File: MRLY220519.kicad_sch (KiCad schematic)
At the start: 2 parts

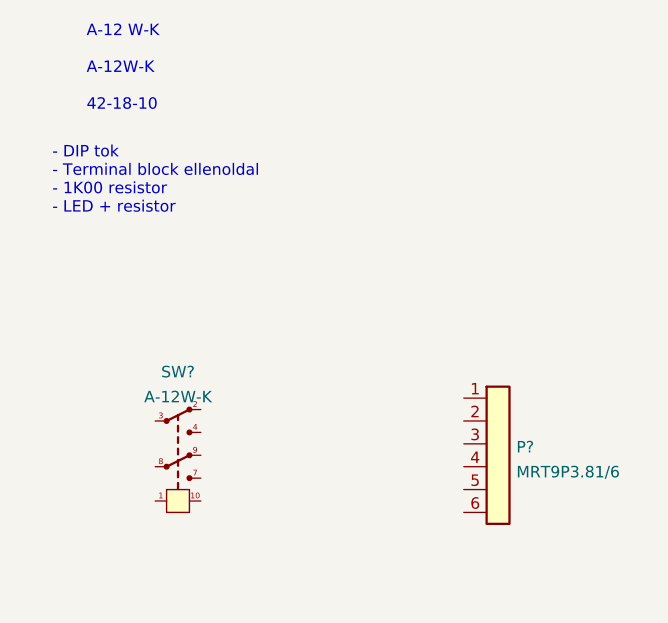
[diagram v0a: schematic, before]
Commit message: updat
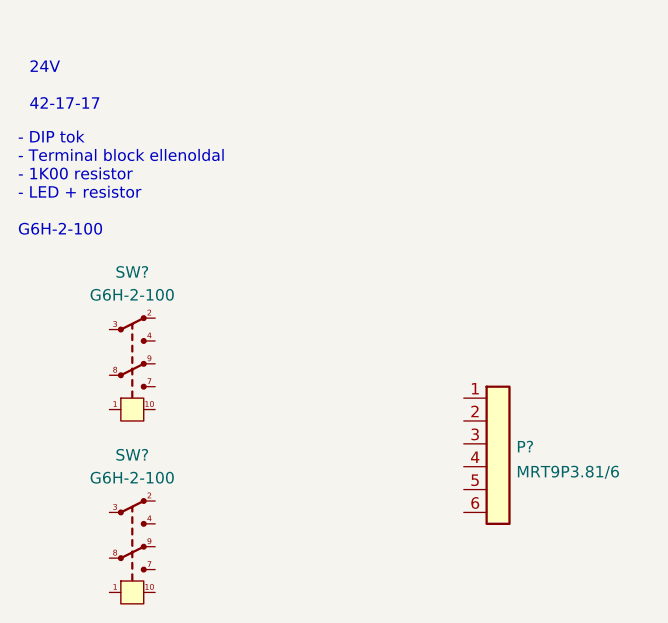
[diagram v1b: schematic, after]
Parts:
- removed SW?: FUJITSU A-12W-K, symbol Switches:FUJITSU A-12W-K
- added SW? (x2): OMRON G6H-2-100, Passive:OMRON G6H-2-100, symbol Switches:OMRON G6H-2-100
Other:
- note added: "- DIP tok - Terminal block ellenoldal - 1K00 resistor - LED + resistor G6H-2-100"
- note added: "24V 42-17-17"
- note removed: "- DIP tok - Terminal block ellenoldal - 1K00 resistor - LED + resistor"
- note removed: "A-12 W-K A-12W-K 42-18-10"
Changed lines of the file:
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@@
 (kicad_sch (version 20211123) (generator eeschema)
   (paper "A4")
-  (text "A-12 W-K\n\nA-12W-K\n\n42-18-10" (at 191.77 30.48 0)
+  (text "\n24V\n\n42-17-17 \n" (at 185.42 30.48 0)
     (effects (font (size 1.27 1.27)) (justify left bottom))
   )
-  (text "- DIP tok\n- Terminal block ellenoldal\n- 1K00 resistor\n- LED + resistor"
-    (at 187.96 41.91 0)
+  (text "- DIP tok\n- Terminal block ellenoldal\n- 1K00 resistor\n- LED + resistor\n\nG6H-2-100"
+    (at 184.15 44.45 0)
     (effects (font (size 1.27 1.27)) (justify left bottom))
+  )
+  (symbol (lib_id "Switches:OMRON G6H-2-100") (at 194.31 74.93 0) (unit 1)
+    (in_bom yes) (on_board yes) (fields_autoplaced)
+    (property "Reference" "SW?" (id 0) (at 196.85 68.58 0))
+    (property "Value" "OMRON G6H-2-100" (id 1) (at 199.39 92.075 0)
+      (effects (font (size 1.27 1.27)) hide)
+    )
+    (property "Footprint" "Passive:OMRON G6H-2-100" (id 2) (at 194.31 67.31 0)
+      (effects (font (size 1.27 1.27)) hide)
+    )
+    (property "Datasheet" "${KNV_DATASHEET}\\AZ850.pdf" (id 3) (at 195.58 93.98 0)
+      (effects (font (size 1.27 1.27)) hide)
+    )
+    (property "Comment" "G6H-2-100" (id 4) (at 196.85 71.12 0))
+    (property "Manufacturer" "FUJITSU;ZETTLER" (id 5) (at 195.58 101.6 0)
+      (effects (font (size 1.27 1.27)) hide)
+    )
+    (property "ManufacturerPartNo" "A-24W-K;AZ850-24;" (id 6) (at 195.58 99.06 0)
+      (effects (font (size 1.27 1.27)) hide)
+    )
+    (property "Supplier" "TME-A-24W-K;TME-AZ850-24;" (id 7) (at 195.58 96.52 0)
+      (effects (font (size 1.27 1.27)) hide)
+    )
+    (pin "1")
+    (pin "10")
+    (pin "2")
+    (pin "3")
+    (pin "4")
+    (pin "7")
+    (pin "8")
+    (pin "9")
   )
   (symbol (lib_id "Connectors:Terminal Block 6 3.81 Straight") (at 236.22 60.96 0) (unit 1)
@@
     (pin "6")
   )
-  (symbol (lib_id "Switches:FUJITSU A-12W-K") (at 199.39 64.77 0) (unit 1)
+  (symbol (lib_id "Switches:OMRON G6H-2-100") (at 194.31 54.61 0) (unit 1)
     (in_bom yes) (on_board yes) (fields_autoplaced)
-    (property "Reference" "SW?" (id 0) (at 201.93 59.3303 0))
-    (property "Value" "FUJITSU A-12W-K" (id 1) (at 204.47 81.915 0)
+    (property "Reference" "SW?" (id 0) (at 196.85 48.26 0))
+    (property "Value" "OMRON G6H-2-100" (id 1) (at 199.39 71.755 0)
       (effects (font (size 1.27 1.27)) hide)
     )
-    (property "Footprint" "" (id 2) (at 199.39 57.15 0)
+    (property "Footprint" "Passive:OMRON G6H-2-100" (id 2) (at 194.31 46.99 0)
       (effects (font (size 1.27 1.27)) hide)
     )
-    (property "Datasheet" "${KNV_DATASHEET}\\5M.pdf" (id 3) (at 200.66 83.82 0)
+    (property "Datasheet" "${KNV_DATASHEET}\\AZ850.pdf" (id 3) (at 195.58 73.66 0)
       (effects (font (size 1.27 1.27)) hide)
     )
-    (property "Comment" "A-12W-K" (id 4) (at 201.93 62.1054 0))
-    (property "Manufacturer" "FUJITSU" (id 5) (at 200.66 91.44 0)
+    (property "Comment" "G6H-2-100" (id 4) (at 196.85 50.8 0))
+    (property "Manufacturer" "FUJITSU;ZETTLER" (id 5) (at 195.58 81.28 0)
       (effects (font (size 1.27 1.27)) hide)
     )
-    (property "ManufacturerPartNo" "A-12W-K;" (id 6) (at 200.66 88.9 0)
+    (property "ManufacturerPartNo" "A-24W-K;AZ850-24;" (id 6) (at 195.58 78.74 0)
       (effects (font (size 1.27 1.27)) hide)
     )
-    (property "Supplier" "TME-A-12W-K;" (id 7) (at 200.66 86.36 0)
+    (property "Supplier" "TME-A-24W-K;TME-AZ850-24;" (id 7) (at 195.58 76.2 0)
       (effects (font (size 1.27 1.27)) hide)
     )
@@
       (reference "P?") (unit 1) (value "Terminal Block 6 3.81 Straight") (footprint "")
     )
-    (path "/aec40859-dddb-4aa7-9566-0d4ab09d1189"
-      (reference "SW?") (unit 1) (value "FUJITSU A-12W-K") (footprint "")
+    (path "/5a83c478-c98d-4120-9ecb-99e35fd2c85e"
+      (reference "SW?") (unit 1) (value "OMRON G6H-2-100") (footprint "Passive:OMRON G6H-2-100")
+    )
+    (path "/c9e3168c-bc1d-46b9-a241-745d3c32565c"
+      (reference "SW?") (unit 1) (value "OMRON G6H-2-100") (footprint "Passive:OMRON G6H-2-100")
     )
   )
